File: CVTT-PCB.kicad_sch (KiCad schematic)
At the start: 66 parts, among them J1 SERVO1, J2 SERVO2, J3 LCD SCREEN, J4 LCD BUTTONS, J5 Conn_ARM_SWD_TagConnect_TC2030, J7 Barrel_Jack, P2 DC2, P5 DC1, P8 STEPPER, Q7 BSS138, Q8 BSS138, SW1 SW_SPST, U2 TPS259474ARPWR, U3 MPM3610GQV-P, U4 TPS62203DBV, U5 STM32G0B1RET6, U7 RASPBERRY PI ZERO 2 W

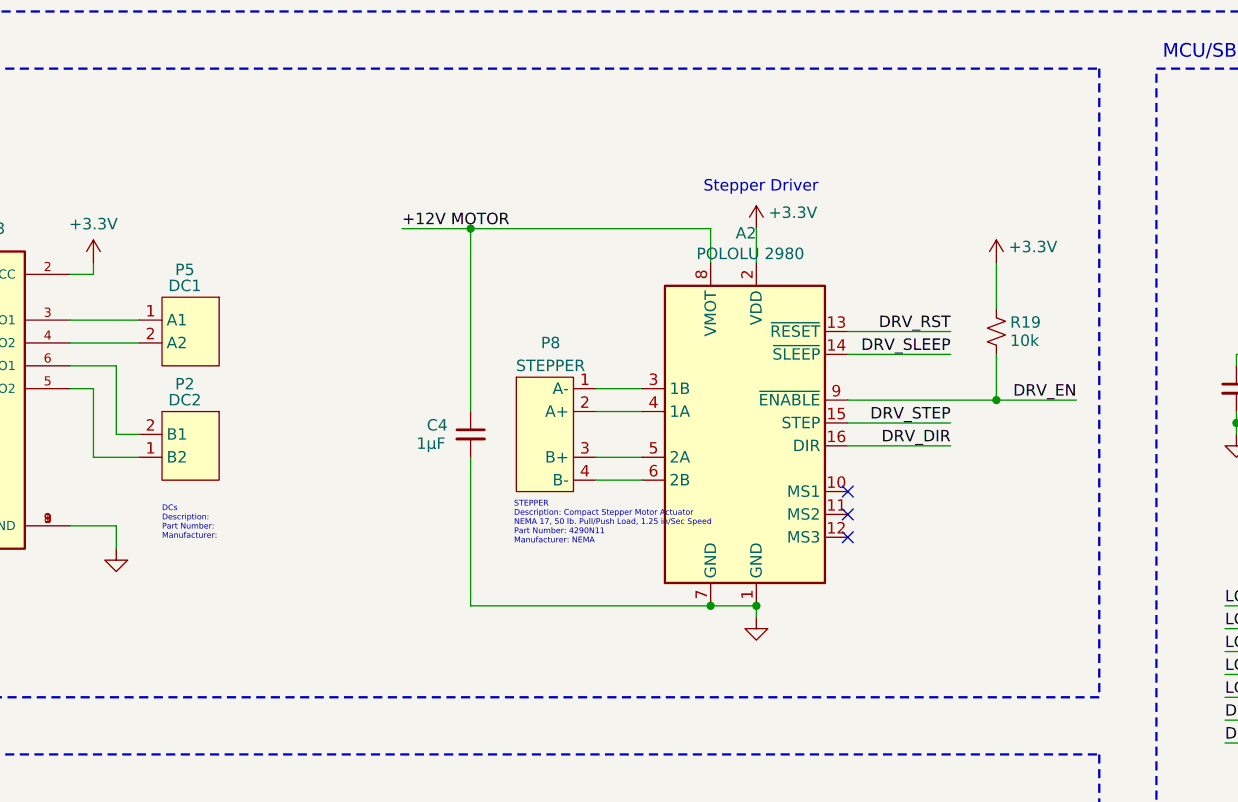
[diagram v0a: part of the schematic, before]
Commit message: update sch info
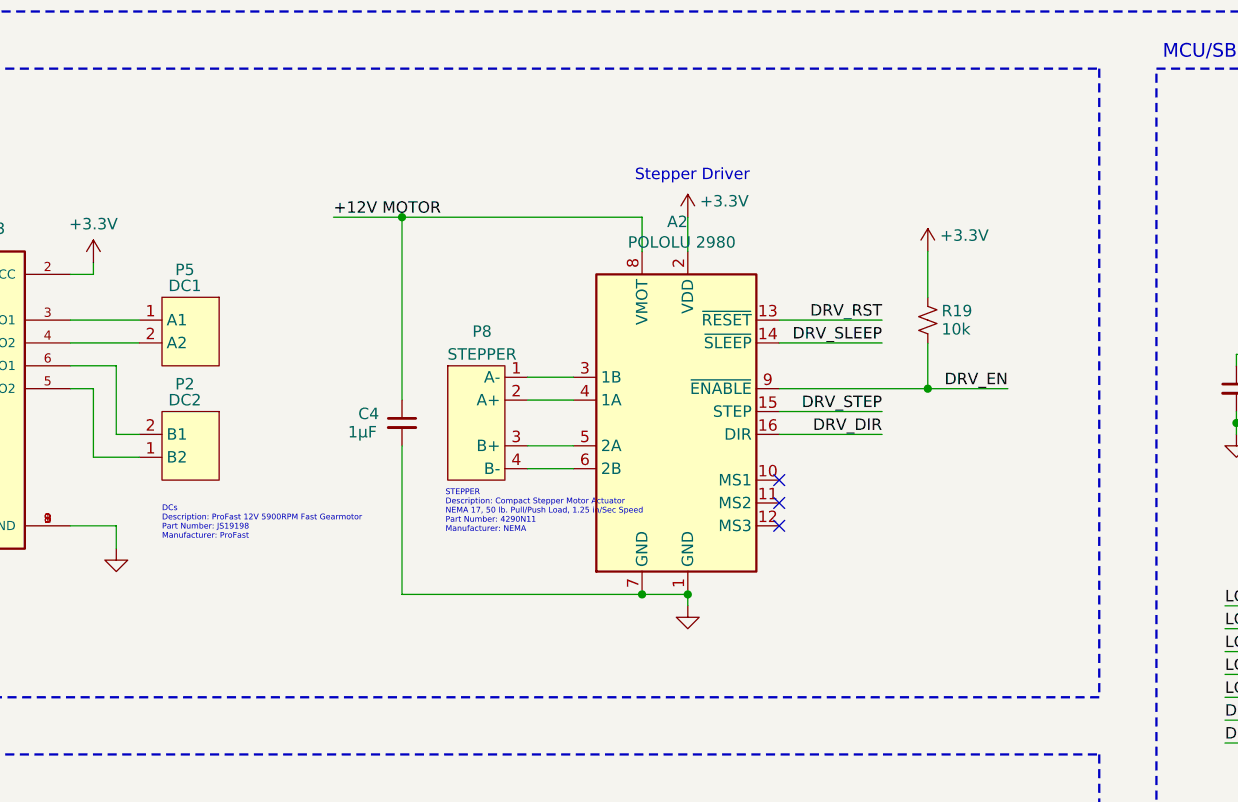
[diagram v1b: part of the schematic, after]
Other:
- note added: "DCs Description: ProFast 12V 5900RPM Fast Gearmotor Part Number: JS19198 Manufacturer: ProFast"
- note removed: "DCs Description: Part Number: Manufacturer:"
- moved on the sheet: A2, C4, P8, R19
